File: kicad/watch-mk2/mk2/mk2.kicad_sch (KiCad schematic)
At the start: 51 parts, among them IC1 MDBT50Q, IC2 M41T62LC6F, J1 Conn_01x10_Female, J2 USB_C_Receptacle_USB2.0, J3 Conn_01x02_Female, J4 503480-0400, J5 Conn_01x02_Female, J6 Conn_01x02_Female, P1 AXT610124, Q3 Si1308EDL, Q4 Si1308EDL, SW1 B5, SW2 B1, SW4 B3, U1 TPS60151DRV, U2 LM3671MF-2.8_NOPB, U3 MCP73831-2-OT, U4 BMA400, U6 MAX17262REWL+T, Y1 32.768kHz

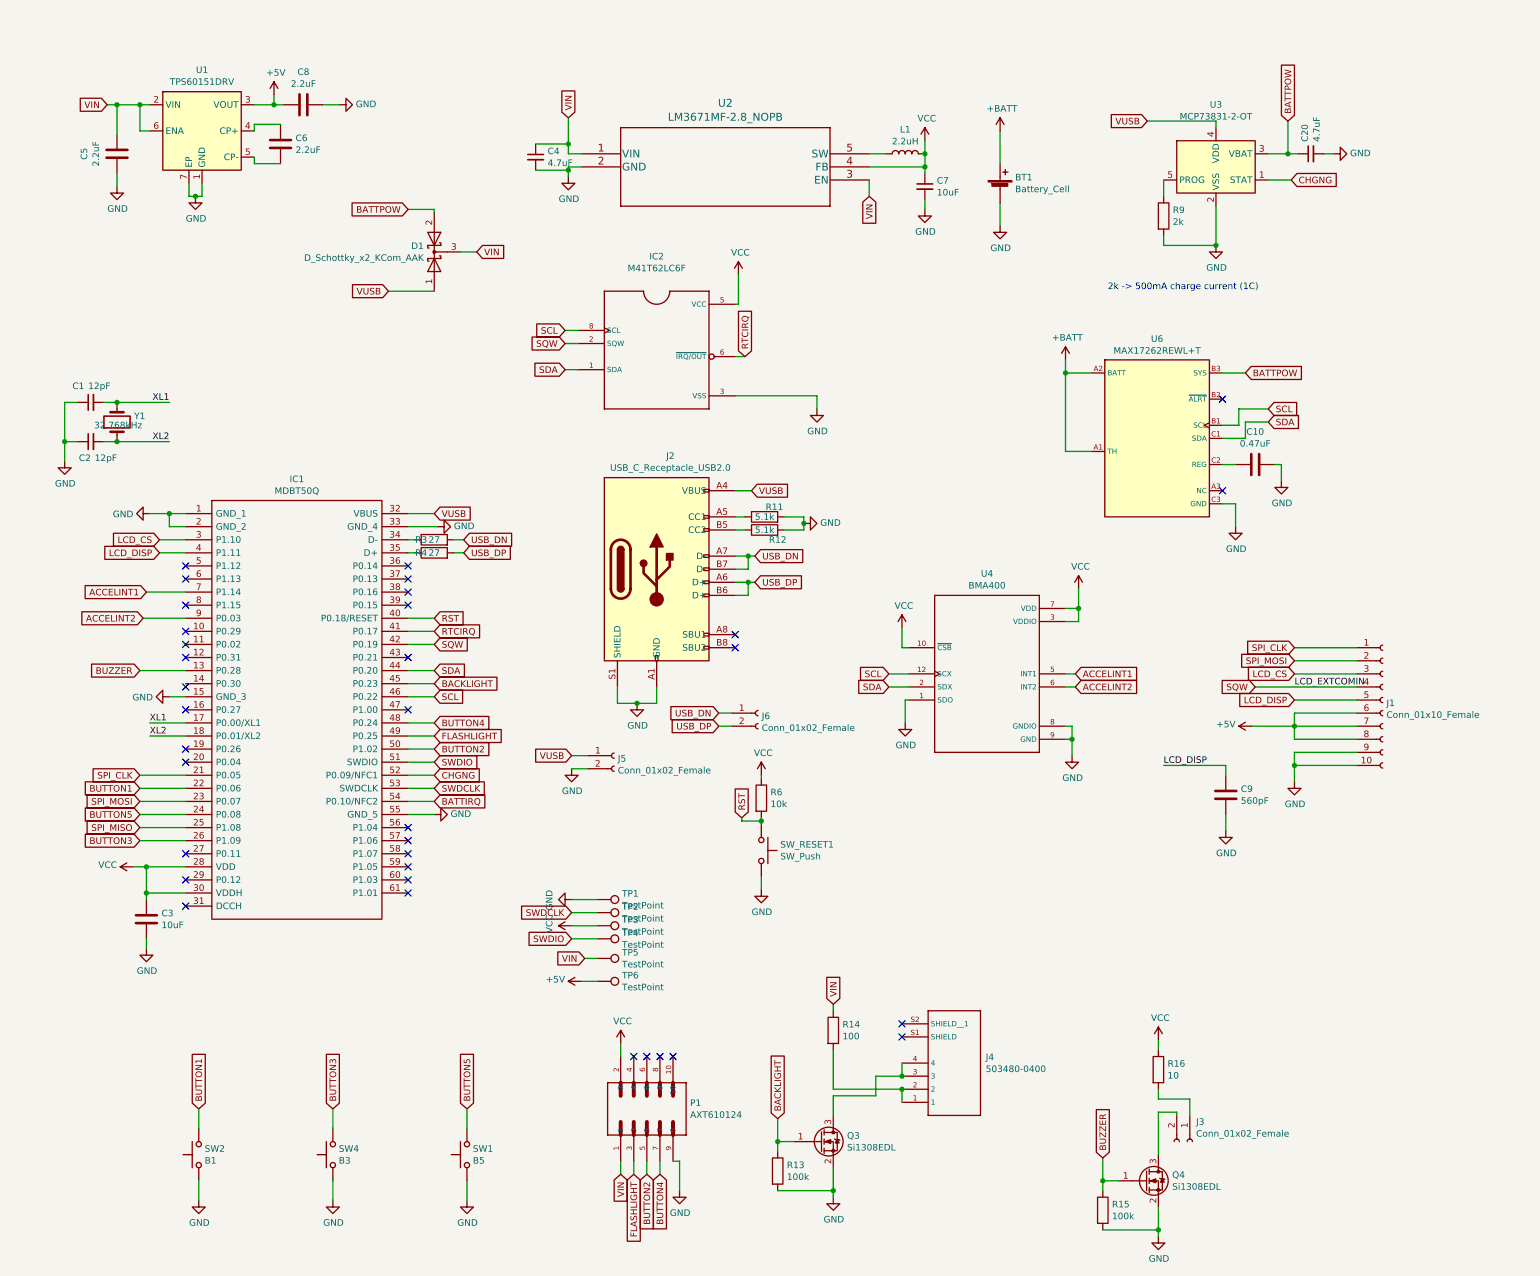
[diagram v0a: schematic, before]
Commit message: checkpoint
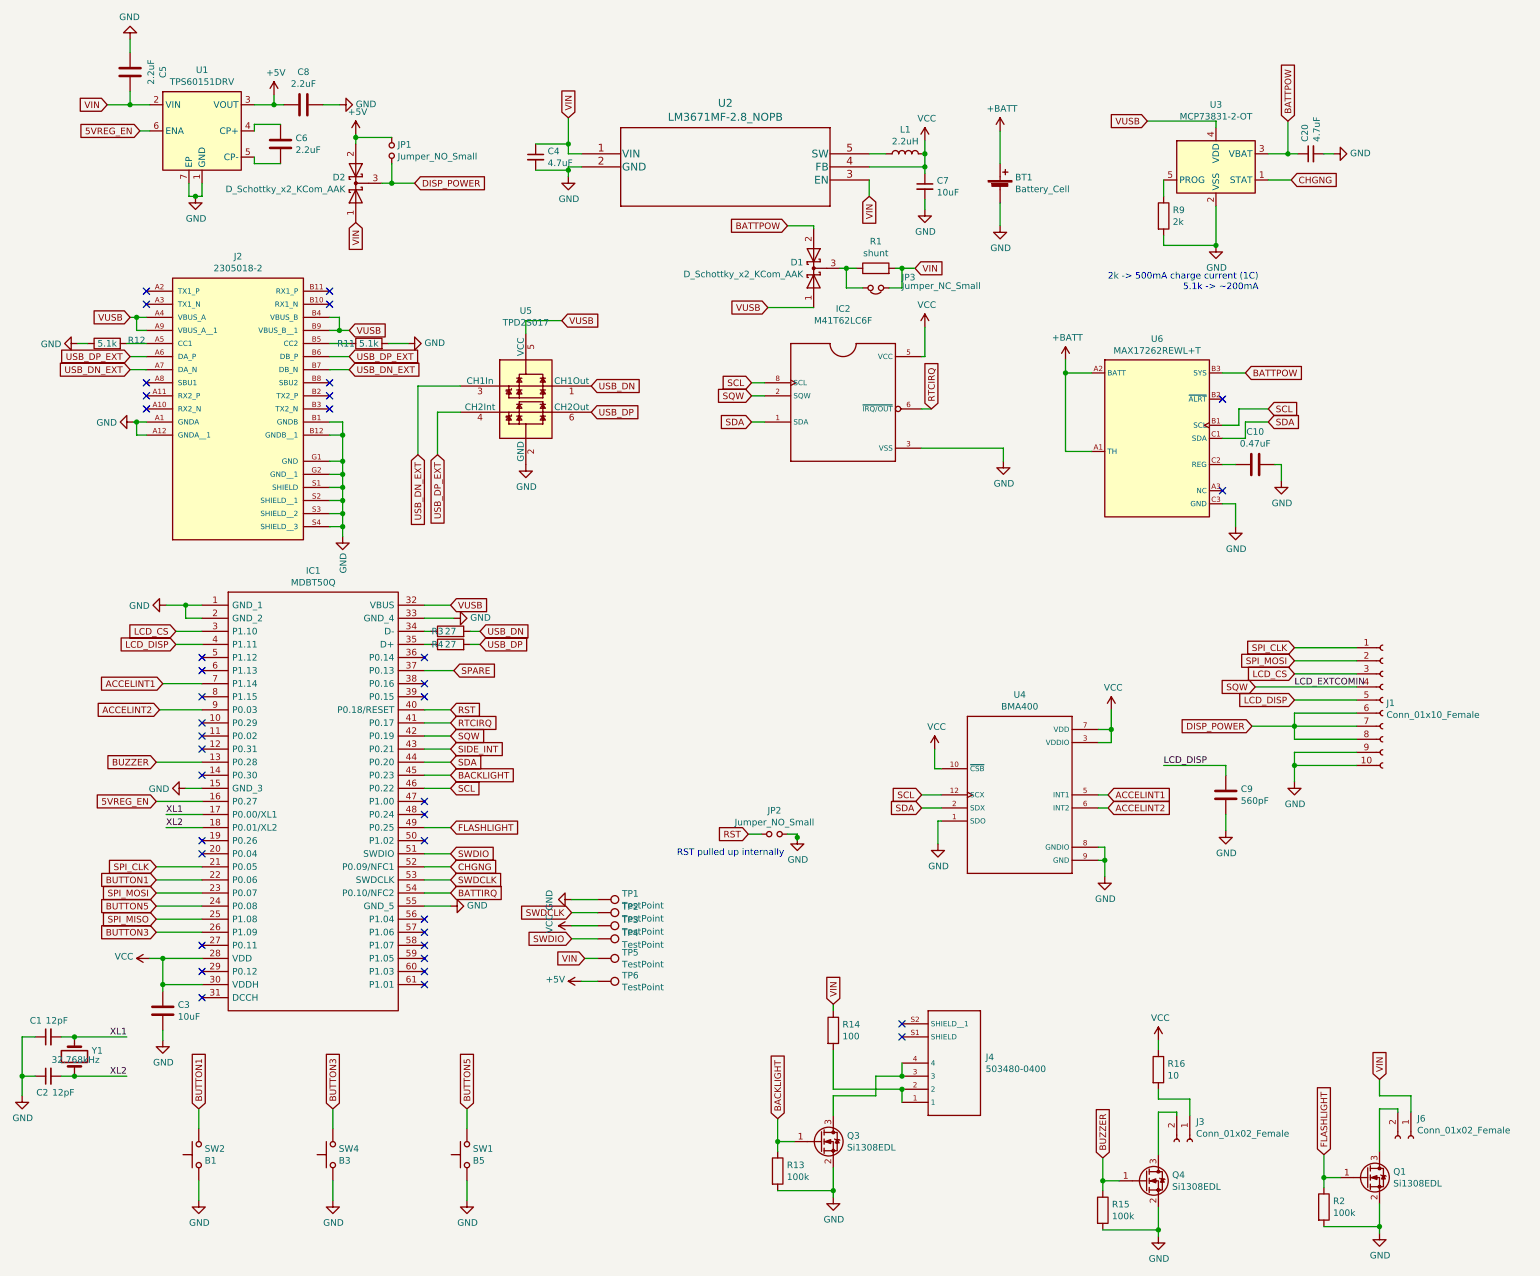
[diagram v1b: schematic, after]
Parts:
- removed J2: USB_C_Receptacle_USB2.0, Connector_USB:USB_C_Receptacle_Palconn_UTC16-G, symbol Connector:USB_C_Receptacle_USB2.0
- removed J5: Conn_01x02_Female, Connector_PinHeader_2.00mm:PinHeader_1x02_P2.00mm_Vertical, symbol Connector:Conn_01x02_Female
- removed P1: AXT610124, libs:PANASONIC_AXT610124, symbol AXT610124:AXT610124
- removed R6: 10k, Resistor_SMD:R_0603_1608Metric_Pad1.05x0.95mm_HandSolder, symbol Device:R
- removed SW_RESET1: SW_Push, Button_Switch_SMD:SW_SPST_CK_KXT3, symbol Switch:SW_Push
- added D2: D_Schottky_x2_KCom_AAK, Package_TO_SOT_SMD:TSOT-23, symbol Device:D_Schottky_x2_KCom_AAK
- added J2: 2305018-2, te-waterproof-usb-2305018-2:TE_2305018-2, symbol 2305018-2:2305018-2
- added JP1, JP2: Jumper_NO_Small, Jumper:SolderJumper-2_P1.3mm_Open_Pad1.0x1.5mm, symbol Device:Jumper_NO_Small
- added JP3: Jumper_NC_Small, Jumper:SolderJumper-2_P1.3mm_Bridged_Pad1.0x1.5mm, symbol Device:Jumper_NC_Small
- added Q1: Si1308EDL, Package_TO_SOT_SMD:SOT-323_SC-70, symbol Device:Q_NMOS_GSD
- added R1: shunt, Resistor_SMD:R_0603_1608Metric, symbol Device:R
- added R2: 100k, Resistor_SMD:R_0603_1608Metric_Pad1.05x0.95mm_HandSolder, symbol Device:R
- added U5: TPD2S017, Package_TO_SOT_SMD:SOT-23-6, symbol Power_Protection:TPD2S017
- J6: footprint Connector_PinHeader_2.00mm:PinHeader_1x02_P2.00mm_Vertical -> Connector_PinSocket_2.00mm:PinSocket_1x02_P2.00mm_Vertical; package (none) -> DNP
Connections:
- net +5V: now also D2.2 (A), JP1.2; no longer J1.6 (Pin_6), J1.7 (Pin_7), J1.8 (Pin_8)
- net FLASHLIGHT: now also Q1.1 (G), R2.1
- net GND: now also R12.1, J2.A1 (GNDA), J2.A12 (GNDA__1), J2.B1 (GNDB), J2.B12 (GNDB__1), J2.G1 (GND), J2.G2 (GND__1), J2.S1 (SHIELD), J2.S2 (SHIELD__1), J2.S3 (SHIELD__2), J2.S4 (SHIELD__3), JP2.2, Q1.2 (S), R2.2, U5.2 (GND); no longer R12.2
- net RST: now also JP2.1
- net USB_DN: now also U5.1 (CH1Out); no longer J6.1 (Pin_1)
- net USB_DP: now also U5.6 (CH2Out); no longer J6.2 (Pin_2)
- net VIN: now also J6.1 (Pin_1), D2.1 (A), JP3.1, R1.2; no longer D1.3 (K), U1.6 (ENA)
- net VUSB: now also J2.A4 (VBUS_A), J2.A9 (VBUS_A__1), J2.B4 (VBUS_B), J2.B9 (VBUS_B__1), U5.5 (VCC)
- net 5VREG_EN: now reaches IC1.16 (P0.27)
- net 5VREG_EN: now also U1.6 (ENA)
- net SPARE: now reaches IC1.37 (P0.13)
- net SIDE_INT: now reaches IC1.43 (P0.21)
- net at R11.1: now also J2.B5 (CC2)
- net BUTTON2: no longer names the net of IC1.50 (P1.02)
- net BUTTON4: no longer names the net of IC1.48 (P0.24)
- new net: J2.A5 (CC1), R12.2
- new net: D1.3 (K), JP3.2, R1.1
- new net: J6.2 (Pin_2), Q1.3 (D)
- new net DISP_POWER: D2.3 (K), J1.6 (Pin_6), J1.7 (Pin_7), J1.8 (Pin_8), JP1.1
- new net USB_DN_EXT: J2.A7 (DA_N), J2.B7 (DB_N), U5.3 (CH1In)
- new net USB_DP_EXT: J2.A6 (DA_P), J2.B6 (DB_P), U5.4 (CH2Int)
- no-connect marks 35 -> 38
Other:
- note added: "2k -> 500mA charge current (1C) 5.1k -> ~~200mA"
- note added: "RST pulled up internally"
- note removed: "2k -> 500mA charge current (1C)"
- moved on the sheet: C1, C2, C3, C5, D1, IC1, IC2, R11, R12, R3, R4, U4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

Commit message: checkpoint
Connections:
- net BATTPOW: no longer D1.2 (A)
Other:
- note added: "2k -> 500mA charge current (1C) 5.1k -> ~200mA"
- note added: "Display and Backlight"
- note added: "I/O"
- note added: "Jeff Cooper - jeff@thejeffcooper.com - Pittsburgh, PA"
- note added: "NOTE: Unclear if this 5V regulator is actually effective at such a low current level"
- note added: "Peripherals"
- note added: "Power and Battery"
- note added: "RTC"
- note added: "Sharp Memory LCD"
- note added: "Test Points"
- note added: "USB"
- note added: "accelerometer"
- note added: "https://hackaday.io/project/169967-nrf52-smartwatch"
- note added: "nRF52840"
- note added: "nRF52840 Smartwatch"
- note removed: "2k -> 500mA charge current (1C) 5.1k -> ~~200mA"
- moved on the sheet: BT1, C1, C10, C2, C20, C3, C4, C5, C6, C7, C8, C9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
